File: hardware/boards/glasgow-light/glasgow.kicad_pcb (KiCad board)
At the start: 2 copper layers, 64 x 20 mm, 172 parts, among them J1 USB_C_USB2.0, J2 IDC-Header_2x5_P2.54mm, J3 IDC-Header_2x5_P2.54mm, U1 LM358_DFN, U10 SN74LVC1T45DCKR, U11 SN74LVC1T45DCKR, U12 INA180A2, U15 TPD3S014, U16 SN74LVC1T45DCKR, U17 SN74LVC1T45DCKR, U18 SN74LVC1T45DCKR, U19 PCA6408APW, U2 GD32VF103T, U31 TPS73101DBV, U36 TLV73312PQDRVR, U4 SN74LVC1T45DCKR, U5 ICE40UP5K-SG48ITR, U6 SN74LVC1T45DCKR, U8 TLV75533PDRVR, U9 SN74LVC1T45DCKR, Y1 8M

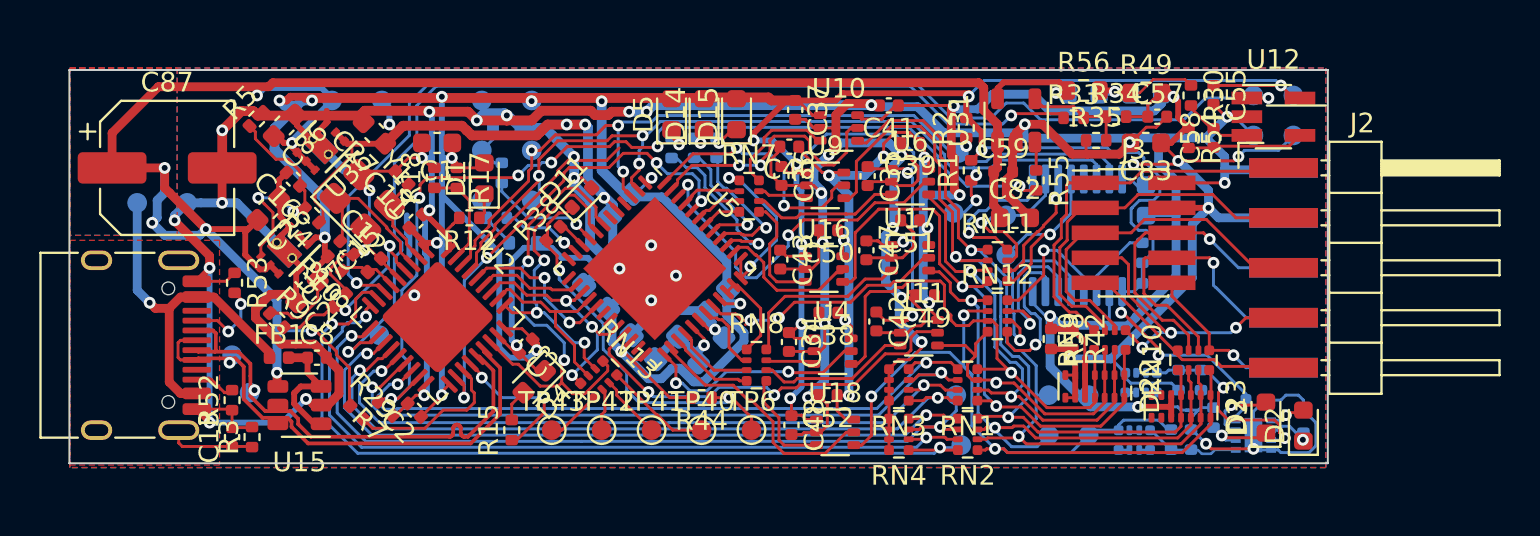
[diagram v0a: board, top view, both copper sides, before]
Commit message: optimize
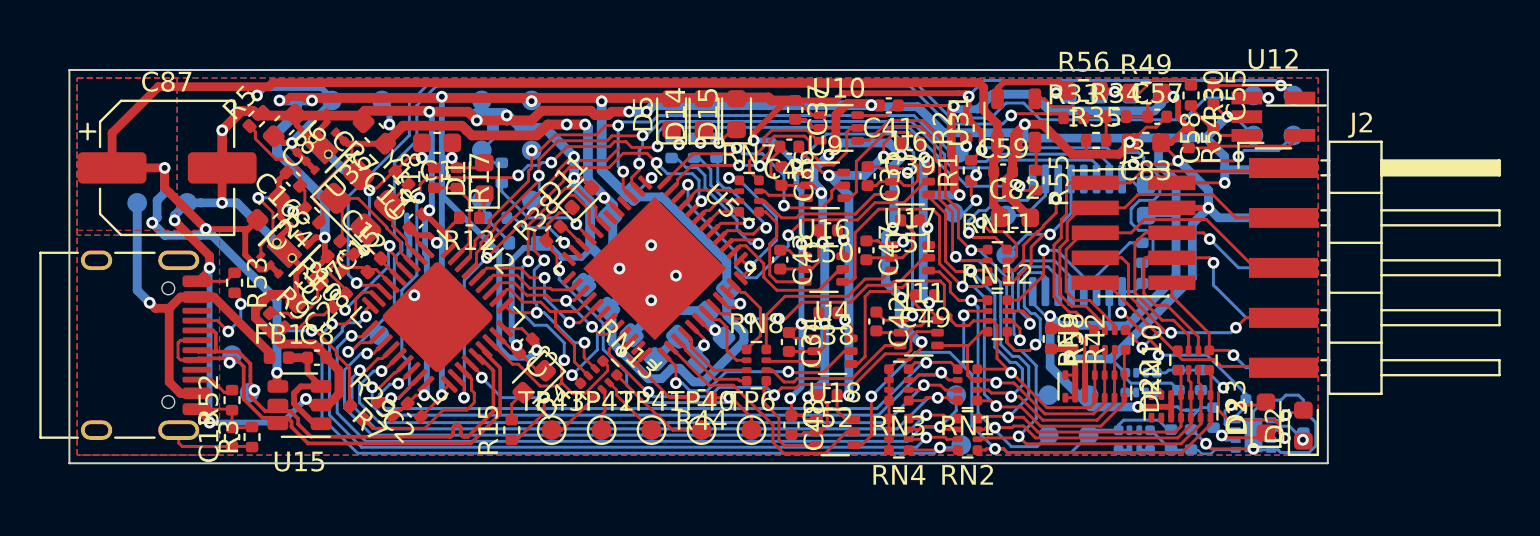
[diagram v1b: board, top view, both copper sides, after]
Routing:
- net GND: track 388.7 -> 387.0 mm
- net +3V3: track 239.6 -> 240.7 mm
- net +5V: track 102.8 -> 103.5 mm
